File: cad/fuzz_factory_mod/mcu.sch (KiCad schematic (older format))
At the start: 16 parts, among them J201 Conn_MCU_SWD, U201 STM32F303VCTx, Y201 Resonator_Small

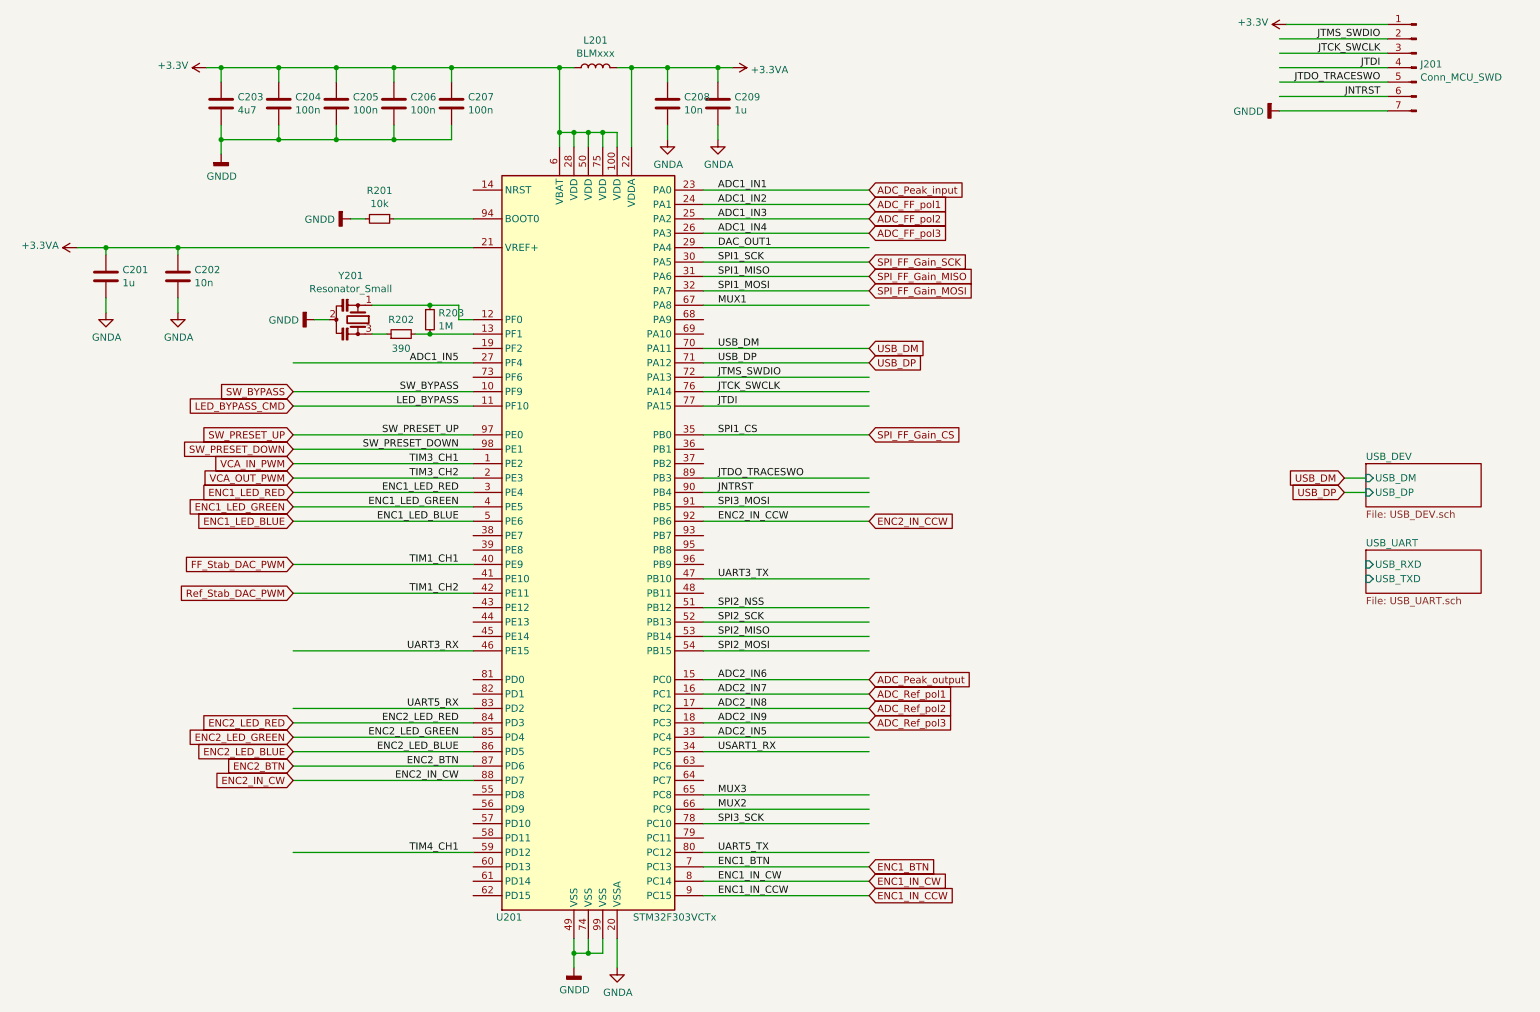
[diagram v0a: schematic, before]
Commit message: Continued schematic.
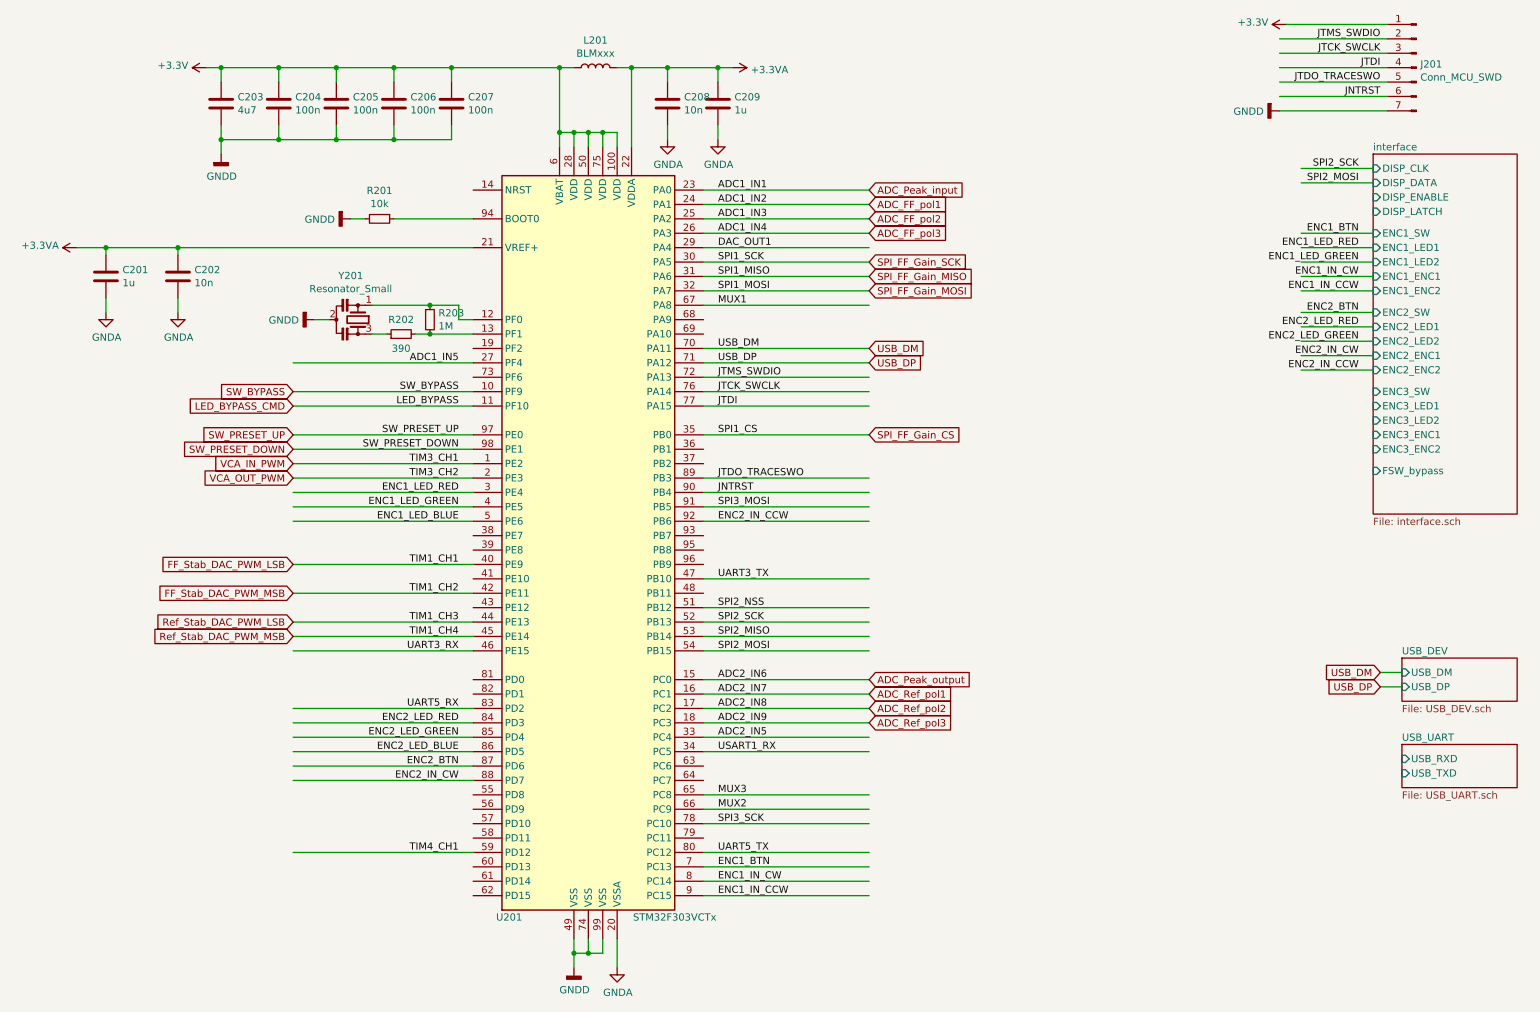
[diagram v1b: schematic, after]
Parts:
- Y201: footprint (none) -> Pin_Headers:Pin_Header_Straight_1x03_Pitch2.54mm
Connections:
- net labels added: FF_Stab_DAC_PWM_LSB, FF_Stab_DAC_PWM_MSB, Ref_Stab_DAC_PWM_LSB, Ref_Stab_DAC_PWM_MSB, TIM1_CH3, TIM1_CH4
- net labels removed: FF_Stab_DAC_PWM, Ref_Stab_DAC_PWM
- wire segments 131 -> 145
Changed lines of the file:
@@
 $Descr A4 11693 8268
 encoding utf-8
-Sheet 2 22
+Sheet 2 26
 Title ""
 Date ""
@@
 F 0 "Y201" V 2645 2600 50  0000 C CNN
 F 1 "Resonator_Small" V 2736 2600 50  0000 C CNN
-F 2 "" H 2925 2650 50  0001 C CNN
+F 2 "Pin_Headers:Pin_Header_Straight_1x03_Pitch2.54mm" H 2925 2650 50  0001 C CNN
 F 3 "~" H 2925 2650 50  0001 C CNN
 	1    2950 2650
@@
 Text GLabel 2500 3550 0    50   Input ~ 0
 SW_PRESET_DOWN
-Text GLabel 2500 3850 0    50   Input ~ 0
-ENC1_LED_RED
-Text GLabel 2500 3950 0    50   Input ~ 0
-ENC1_LED_GREEN
-Text GLabel 2500 4050 0    50   Input ~ 0
-ENC1_LED_BLUE
-Text GLabel 2500 5450 0    50   Input ~ 0
-ENC2_LED_RED
-Text GLabel 2500 5550 0    50   Input ~ 0
-ENC2_LED_GREEN
-Text GLabel 2500 5650 0    50   Input ~ 0
-ENC2_LED_BLUE
-Text GLabel 2500 5750 0    50   Input ~ 0
-ENC2_BTN
-Text GLabel 2500 5850 0    50   Input ~ 0
-ENC2_IN_CW
-Text GLabel 6500 6550 2    50   Input ~ 0
-ENC1_IN_CW
-Text GLabel 6500 6650 2    50   Input ~ 0
-ENC1_IN_CCW
-Text GLabel 6500 6450 2    50   Input ~ 0
-ENC1_BTN
-Text GLabel 6500 4050 2    50   Input ~ 0
-ENC2_IN_CCW
 Text GLabel 2500 3650 0    50   Input ~ 0
 VCA_IN_PWM
@@
 VCA_OUT_PWM
 Text GLabel 2500 4350 0    50   Input ~ 0
-FF_Stab_DAC_PWM
-Text GLabel 2500 4550 0    50   Input ~ 0
-Ref_Stab_DAC_PWM
+FF_Stab_DAC_PWM_LSB
+Text GLabel 2500 4750 0    50   Input ~ 0
+Ref_Stab_DAC_PWM_LSB
 $Sheet
-S 9950 4250 800  300
+S 10200 5600 800  300
 U 5EB00B3E
 F0 "USB_UART" 50
 F1 "USB_UART.sch" 50
-F2 "USB_RXD" I L 9950 4350 50
-F3 "USB_TXD" I L 9950 4450 50
+F2 "USB_RXD" I L 10200 5700 50
+F3 "USB_TXD" I L 10200 5800 50
 $EndSheet
 $Sheet
-S 9950 3650 800  300
+S 10200 5000 800  300
 U 5EB591ED
 F0 "USB_DEV" 50
 F1 "USB_DEV.sch" 50
-F2 "USB_DM" I L 9950 3750 50
-F3 "USB_DP" I L 9950 3850 50
+F2 "USB_DM" I L 10200 5100 50
+F3 "USB_DP" I L 10200 5200 50
 $EndSheet
-Text GLabel 9800 3750 0    50   Input ~ 0
+Text GLabel 10050 5100 0    50   Input ~ 0
 USB_DM
-Text GLabel 9800 3850 0    50   Input ~ 0
+Text GLabel 10050 5200 0    50   Input ~ 0
 USB_DP
 Wire Wire Line
-	9800 3750 9950 3750
-Wire Wire Line
-	9950 3850 9800 3850
+	10050 5100 10200 5100
+Wire Wire Line
+	10200 5200 10050 5200
+Text Label 3650 4750 2    50   ~ 0
+TIM1_CH3
+Text Label 3650 4850 2    50   ~ 0
+TIM1_CH4
+Wire Wire Line
+	3750 4750 2500 4750
+Wire Wire Line
+	3750 4850 2500 4850
+Text GLabel 2500 4550 0    50   Input ~ 0
+FF_Stab_DAC_PWM_MSB
+Text GLabel 2500 4850 0    50   Input ~ 0
+Ref_Stab_DAC_PWM_MSB
+$Sheet
+S 10000 1500 1000 2500
+U 5EEFDD5E
+F0 "interface" 50
+F1 "interface.sch" 50
+F2 "DISP_CLK" I L 10000 1600 50
+F3 "DISP_DATA" I L 10000 1700 50
+F4 "DISP_ENABLE" I L 10000 1800 50
+F5 "DISP_LATCH" I L 10000 1900 50
+F6 "ENC1_SW" I L 10000 2050 50
+F7 "ENC1_LED1" I L 10000 2150 50
+F8 "ENC1_LED2" I L 10000 2250 50
+F9 "ENC1_ENC1" I L 10000 2350 50
+F10 "ENC1_ENC2" I L 10000 2450 50
+F11 "FSW_bypass" I L 10000 3700 50
+F12 "ENC2_SW" I L 10000 2600 50
+F13 "ENC2_LED1" I L 10000 2700 50
+F14 "ENC2_LED2" I L 10000 2800 50
+F15 "ENC2_ENC1" I L 10000 2900 50
+F16 "ENC2_ENC2" I L 10000 3000 50
+F17 "ENC3_SW" I L 10000 3150 50
+F18 "ENC3_LED1" I L 10000 3250 50
+F19 "ENC3_LED2" I L 10000 3350 50
+F20 "ENC3_ENC1" I L 10000 3450 50
+F21 "ENC3_ENC2" I L 10000 3550 50
+$EndSheet
+Text Label 9900 1600 2    50   ~ 0
+SPI2_SCK
+Text Label 9900 1700 2    50   ~ 0
+SPI2_MOSI
+Wire Wire Line
+	10000 1600 9500 1600
+Wire Wire Line
+	10000 1700 9500 1700
+Text Label 9900 2700 2    50   ~ 0
+ENC2_LED_RED
+Text Label 9900 2800 2    50   ~ 0
+ENC2_LED_GREEN
+Text Label 9900 2600 2    50   ~ 0
+ENC2_BTN
+Text Label 9900 2900 2    50   ~ 0
+ENC2_IN_CW
+Text Label 9900 2050 2    50   ~ 0
+ENC1_BTN
+Text Label 9900 2350 2    50   ~ 0
+ENC1_IN_CW
+Text Label 9900 2450 2    50   ~ 0
+ENC1_IN_CCW
+Text Label 9900 2150 2    50   ~ 0
+ENC1_LED_RED
+Text Label 9900 2250 2    50   ~ 0
+ENC1_LED_GREEN
+Text Label 9900 3000 2    50   ~ 0
+ENC2_IN_CCW
+Wire Wire Line
+	10000 2050 9500 2050
+Wire Wire Line
+	10000 2150 9500 2150
+Wire Wire Line
+	10000 2250 9500 2250
+Wire Wire Line
+	10000 2350 9500 2350
+Wire Wire Line
+	10000 2450 9500 2450
+Wire Wire Line
+	10000 2600 9500 2600
+Wire Wire Line
+	10000 2700 9500 2700
+Wire Wire Line
+	10000 2800 9500 2800
+Wire Wire Line
+	10000 2900 9500 2900
+Wire Wire Line
+	10000 3000 9500 3000
 $EndSCHEMATC

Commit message: Continued schematic.
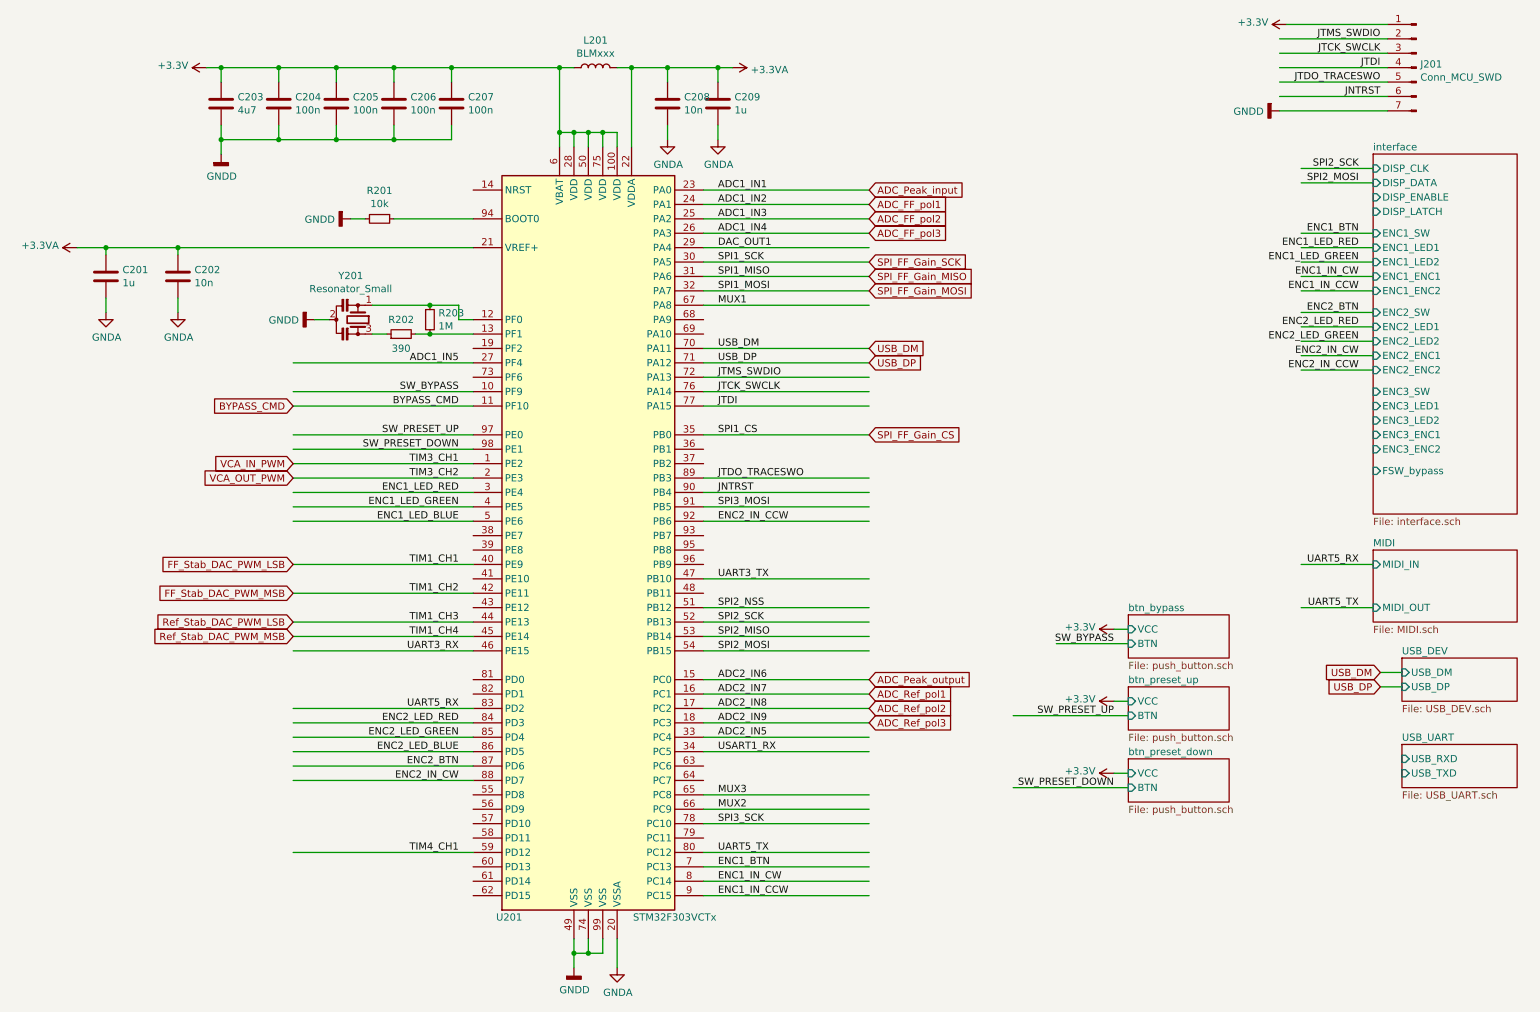
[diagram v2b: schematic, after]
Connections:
- net labels added: BYPASS_CMD
- net labels removed: LED_BYPASS, LED_BYPASS_CMD
- wire segments 145 -> 153
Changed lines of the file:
@@
 $Descr A4 11693 8268
 encoding utf-8
-Sheet 2 26
+Sheet 2 30
 Title ""
 Date ""
@@
 	6500 5450 5350 5450
 Text Label 3650 3250 2    50   ~ 0
-LED_BYPASS
+BYPASS_CMD
 Wire Wire Line
 	3750 3250 2500 3250
@@
 Text GLabel 6500 3450 2    50   Input ~ 0
 SPI_FF_Gain_CS
-Text GLabel 2500 3150 0    50   Input ~ 0
-SW_BYPASS
 Text GLabel 2500 3250 0    50   Input ~ 0
-LED_BYPASS_CMD
-Text GLabel 2500 3450 0    50   Input ~ 0
-SW_PRESET_UP
-Text GLabel 2500 3550 0    50   Input ~ 0
-SW_PRESET_DOWN
+BYPASS_CMD
 Text GLabel 2500 3650 0    50   Input ~ 0
 VCA_IN_PWM
@@
 Wire Wire Line
 	10000 3000 9500 3000
+$Sheet
+S 10000 4250 1000 500
+U 5ECAAB94
+F0 "MIDI" 50
+F1 "MIDI.sch" 50
+F2 "MIDI_IN" I L 10000 4350 50
+F3 "MIDI_OUT" I L 10000 4650 50
+$EndSheet
+Text Label 9900 4350 2    50   ~ 0
+UART5_RX
+Text Label 9900 4650 2    50   ~ 0
+UART5_TX
+Wire Wire Line
+	10000 4350 9500 4350
+Wire Wire Line
+	10000 4650 9500 4650
+$Sheet
+S 8300 4700 700  300
+U 5ED0E0D0
+F0 "btn_bypass" 50
+F1 "push_button.sch" 50
+F2 "BTN" I L 8300 4900 50
+F3 "VCC" I L 8300 4800 50
+$EndSheet
+$Comp
+L power:+3.3V #PWR0229
+U 1 1 5ED10A5A
+P 8200 4800
+F 0 "#PWR0229" H 8200 4650 50  0001 C CNN
+F 1 "+3.3V" V 8215 4928 50  0000 L CNN
+F 2 "" H 8200 4800 50  0001 C CNN
+F 3 "" H 8200 4800 50  0001 C CNN
+	1    8200 4800
+	0    -1   -1   0
+$EndComp
+Wire Wire Line
+	8300 4800 8200 4800
+Text Label 8200 4900 2    50   ~ 0
+SW_BYPASS
+Wire Wire Line
+	8300 4900 7800 4900
+Text Label 8200 5400 2    50   ~ 0
+SW_PRESET_UP
+$Sheet
+S 8300 5200 700  300
+U 5ED20AFC
+F0 "btn_preset_up" 50
+F1 "push_button.sch" 50
+F2 "BTN" I L 8300 5400 50
+F3 "VCC" I L 8300 5300 50
+$EndSheet
+$Sheet
+S 8300 5700 700  300
+U 5ED214FE
+F0 "btn_preset_down" 50
+F1 "push_button.sch" 50
+F2 "BTN" I L 8300 5900 50
+F3 "VCC" I L 8300 5800 50
+$EndSheet
+Text Label 8200 5900 2    50   ~ 0
+SW_PRESET_DOWN
+Wire Wire Line
+	8300 5400 7500 5400
+Wire Wire Line
+	8300 5900 7500 5900
+$Comp
+L power:+3.3V #PWR0230
+U 1 1 5ED48B6A
+P 8200 5300
+F 0 "#PWR0230" H 8200 5150 50  0001 C CNN
+F 1 "+3.3V" V 8215 5428 50  0000 L CNN
+F 2 "" H 8200 5300 50  0001 C CNN
+F 3 "" H 8200 5300 50  0001 C CNN
+	1    8200 5300
+	0    -1   -1   0
+$EndComp
+$Comp
+L power:+3.3V #PWR0231
+U 1 1 5ED48FD7
+P 8200 5800
+F 0 "#PWR0231" H 8200 5650 50  0001 C CNN
+F 1 "+3.3V" V 8215 5928 50  0000 L CNN
+F 2 "" H 8200 5800 50  0001 C CNN
+F 3 "" H 8200 5800 50  0001 C CNN
+	1    8200 5800
+	0    -1   -1   0
+$EndComp
+Wire Wire Line
+	8300 5800 8200 5800
+Wire Wire Line
+	8300 5300 8200 5300
 $EndSCHEMATC
